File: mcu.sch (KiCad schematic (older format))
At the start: 34 parts, among them J17 Conn_01x01_Male, Q6 MMBT5551, U17 UCC27517, U3 STM32F103RCT, X1 8MHz 2520

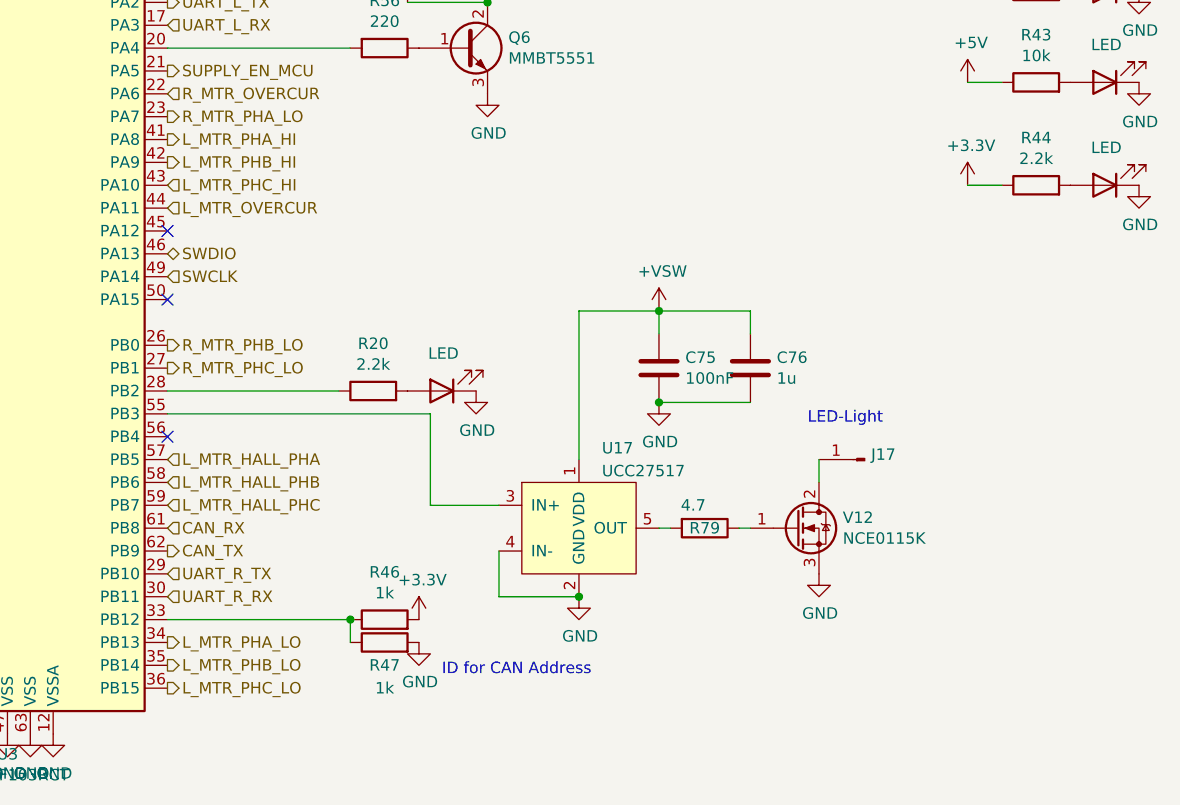
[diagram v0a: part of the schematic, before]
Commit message: Added emergency-break connector
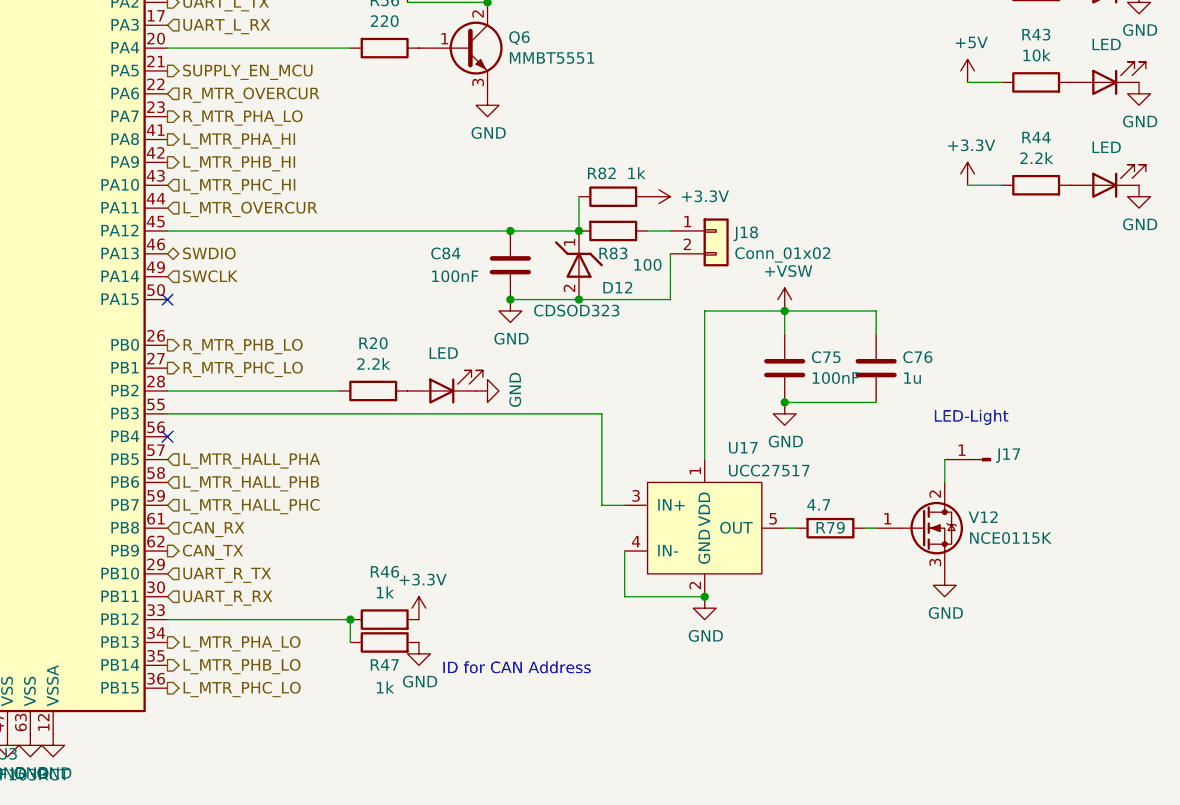
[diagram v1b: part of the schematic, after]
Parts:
- added C84: 100nF, Capacitor_SMD:C_0603_1608Metric, symbol Device:C
- added D12: CDSOD323, Diode_SMD:D_SOD-323, symbol input-board:CDSOD323-boardcomputer
- added J18: Conn_01x02, Connector_Molex:Molex_PicoBlade_53047-0210_1x02_P1.25mm_Vertical, symbol Connector_Generic:Conn_01x02
- added R82: 1k, Resistor_SMD:R_0603_1608Metric, symbol Device:R
- added R83: 100, Resistor_SMD:R_0603_1608Metric, symbol Device:R
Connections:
- net +3V3: now also R82.2
- net GND: now also C84.2, D12.2 (A), J18.2 (Pin_2)
- net at U3.45 (PA12): now also C84.1, D12.1 (K), R82.1, R83.2
- new net: J18.1 (Pin_1), R83.1
- no-connect marks 10 -> 9
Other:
- moved on the sheet: C75, C76, J17, R79, U17, V12
